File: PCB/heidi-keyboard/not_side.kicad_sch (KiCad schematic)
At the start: 65 parts, among them J1 USB_C_Receptacle_USB2.0_14P, J3 AudioJack4, SW1 SW_Push, SW11 SW_Push, SW13 SW_Push, SW14 SW_Push, SW15 SW_Push, SW16 SW_Push, SW17 SW_Push, SW18 SW_Push, SW25 SW_Push, SW26 SW_Push, SW27 SW_Push, SW28 SW_Push, SW29 SW_Push, SW3 SW_Push, SW30 SW_Push, SW37 SW_Push, SW38 SW_Push, SW39 SW_Push, SW40 SW_Push, SW41 SW_Push, SW42 SW_Push, SW49 SW_Push, SW5 SW_Push, SW50 SW_Push, SW51 SW_Push, SW52 SW_Push, SW53 SW_Push, SW54 SW_Push, SW7 SW_Push, SW9 SW_Push

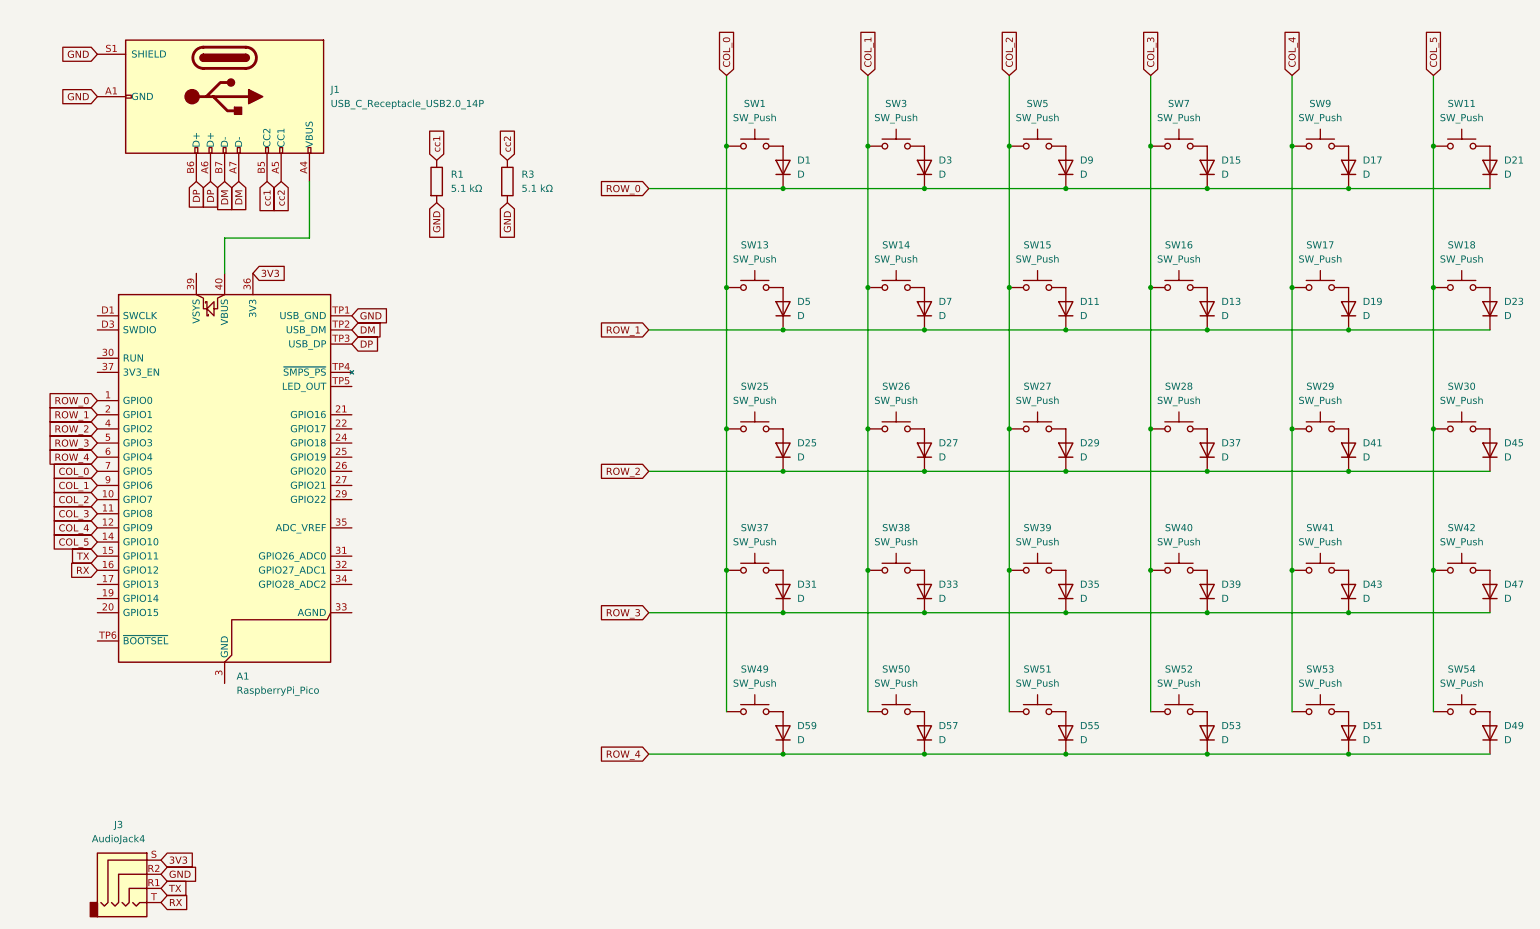
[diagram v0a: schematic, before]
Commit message: aaaaaaaaaaaaaaaaa
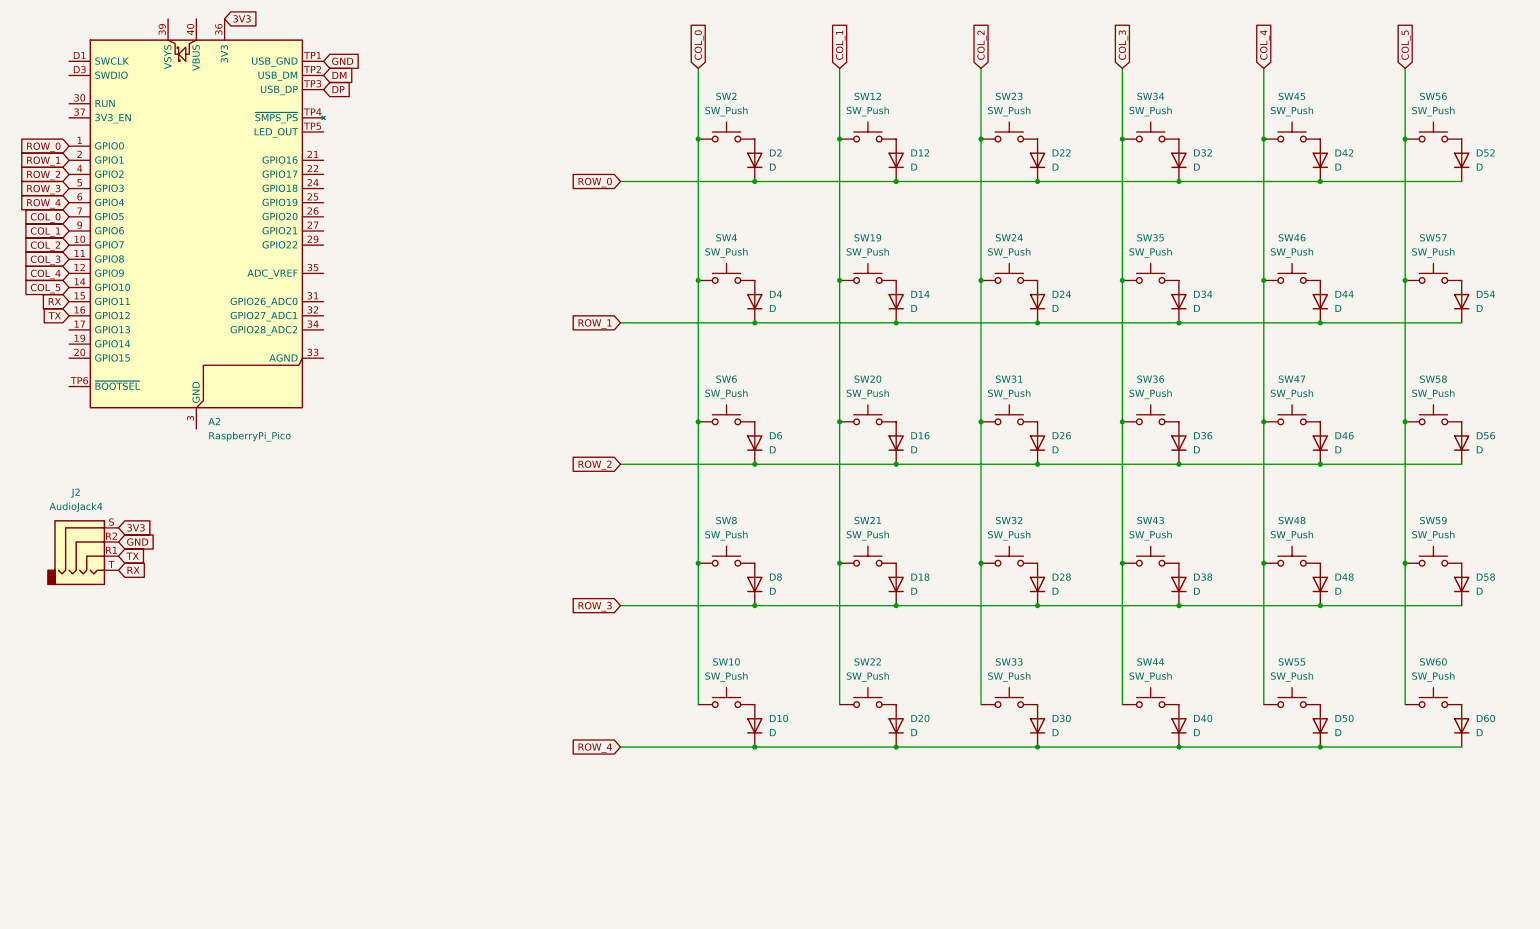
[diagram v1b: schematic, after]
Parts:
- removed A1: RaspberryPi_Pico, Module:RaspberryPi_Pico_SMD, symbol MCU_Module:RaspberryPi_Pico_Extensive
- removed D1, D11, D13, D15, D17, D19, D21, D23, D25, D27, D29, D3, D31, D33, D35, D37, D39, D41, D43, D45, D47, D49, D5, D51, D53, D55, D57, D59, D7, D9: D, symbol Device:D
- removed J1: USB_C_Receptacle_USB2.0_14P, symbol Connector:USB_C_Receptacle_USB2.0_14P
- removed J3: AudioJack4, symbol Connector_Audio:AudioJack4
- removed R1, R3: 5.1 kΩ, symbol Device:R
- removed SW1, SW11, SW13, SW14, SW15, SW16, SW17, SW18, SW25, SW26, SW27, SW28, SW29, SW3, SW30, SW37, SW38, SW39, SW40, SW41, SW42, SW49, SW5, SW50, SW51, SW52, SW53, SW54, SW7, SW9: SW_Push, symbol Switch:SW_Push
- added A2: RaspberryPi_Pico, Module:RaspberryPi_Pico_SMD, symbol MCU_Module:RaspberryPi_Pico_Extensive
- added D10, D12, D14, D16, D18, D2, D20, D22, D24, D26, D28, D30, D32, D34, D36, D38, D4, D40, D42, D44, D46, D48, D50, D52, D54, D56, D58, D6, D60, D8: D, symbol Device:D
- added J2: AudioJack4, symbol Connector_Audio:AudioJack4
- added SW10, SW12, SW19, SW2, SW20, SW21, SW22, SW23, SW24, SW31, SW32, SW33, SW34, SW35, SW36, SW4, SW43, SW44, SW45, SW46, SW47, SW48, SW55, SW56, SW57, SW58, SW59, SW6, SW60, SW8: SW_Push, symbol Switch:SW_Push
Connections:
- net 3V3: now also A2.36 (3V3), J2.S
- net COL_0: now also A2.7 (GPIO5), SW10.1, SW2.1, SW4.1, SW6.1, SW8.1
- net COL_1: now also A2.9 (GPIO6), SW12.1, SW19.1, SW20.1, SW21.1, SW22.1
- net COL_2: now also A2.10 (GPIO7), SW23.1, SW24.1, SW31.1, SW32.1, SW33.1
- net COL_3: now also A2.11 (GPIO8), SW34.1, SW35.1, SW36.1, SW43.1, SW44.1
- net COL_4: now also A2.12 (GPIO9), SW45.1, SW46.1, SW47.1, SW48.1, SW55.1
- net COL_5: now also A2.14 (GPIO10), SW56.1, SW57.1, SW58.1, SW59.1, SW60.1
- net DM: now also A2.TP2 (USB_DM)
- net DP: now also A2.TP3 (USB_DP)
- net GND: now also A2.TP1 (USB_GND), J2.R2
- net ROW_0: now also A2.1 (GPIO0), D12.1 (K), D2.1 (K), D22.1 (K), D32.1 (K), D42.1 (K), D52.1 (K)
- net ROW_1: now also A2.2 (GPIO1), D14.1 (K), D24.1 (K), D34.1 (K), D4.1 (K), D44.1 (K), D54.1 (K)
- net ROW_2: now also A2.4 (GPIO2), D16.1 (K), D26.1 (K), D36.1 (K), D46.1 (K), D56.1 (K), D6.1 (K)
- net ROW_3: now also A2.5 (GPIO3), D18.1 (K), D28.1 (K), D38.1 (K), D48.1 (K), D58.1 (K), D8.1 (K)
- net ROW_4: now also A2.6 (GPIO4), D10.1 (K), D20.1 (K), D30.1 (K), D40.1 (K), D50.1 (K), D60.1 (K)
- net RX: now also A2.15 (GPIO11), J2.T
- net TX: now also A2.16 (GPIO12), J2.R1
- new net: D22.2 (A), SW23.2
- new net: D44.2 (A), SW46.2
- new net: D4.2 (A), SW4.2
- new net: D26.2 (A), SW31.2
- new net: D16.2 (A), SW20.2
- new net: D32.2 (A), SW34.2
- new net: D28.2 (A), SW32.2
- new net: D20.2 (A), SW22.2
- new net: D8.2 (A), SW8.2
- new net: D6.2 (A), SW6.2
- new net: D12.2 (A), SW12.2
- new net: D36.2 (A), SW36.2
- new net: D30.2 (A), SW33.2
- new net: D54.2 (A), SW57.2
- new net: D24.2 (A), SW24.2
- new net: D60.2 (A), SW60.2
- new net: D18.2 (A), SW21.2
- new net: D10.2 (A), SW10.2
- new net: D50.2 (A), SW55.2
- new net: D34.2 (A), SW35.2
- new net: D58.2 (A), SW59.2
- new net: D38.2 (A), SW43.2
- new net: D52.2 (A), SW56.2
- new net: D42.2 (A), SW45.2
- new net: D46.2 (A), SW47.2
- new net: D14.2 (A), SW19.2
- new net: D48.2 (A), SW48.2
- new net: D56.2 (A), SW58.2
- new net: D2.2 (A), SW2.2
- new net: D40.2 (A), SW44.2
- new net: A2.13 (GND), A2.18 (GND), A2.23 (GND), A2.28 (GND), A2.3 (GND), A2.38 (GND), A2.8 (GND), A2.D2 (GND)

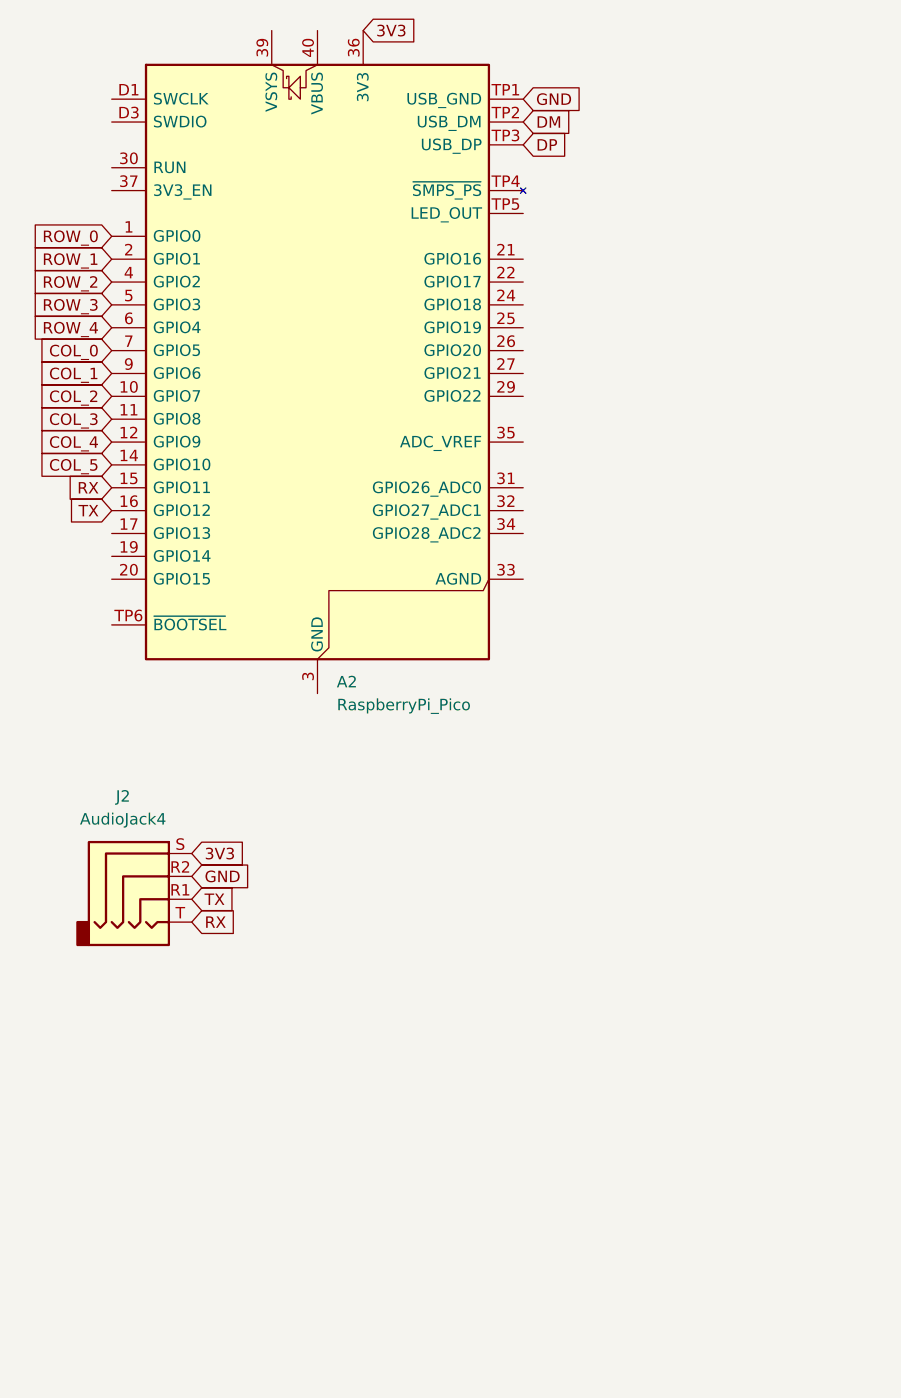
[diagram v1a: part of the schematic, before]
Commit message: aaaaaaaaaaaaaaaa
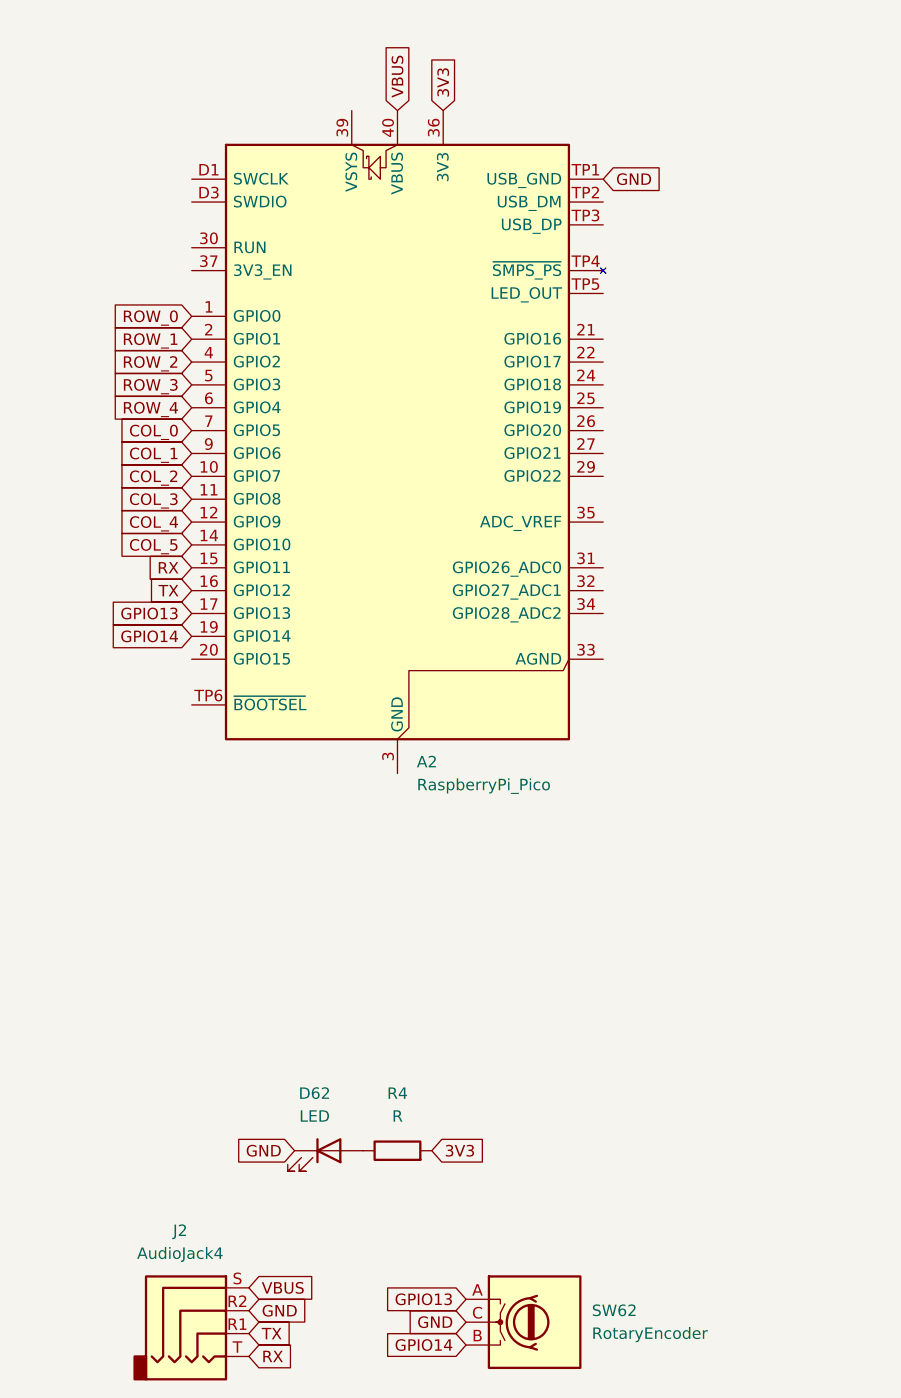
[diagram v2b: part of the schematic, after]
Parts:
- added D62: LED, symbol Device:LED
- added R4: R, symbol Device:R
- added SW62: RotaryEncoder, symbol Device:RotaryEncoder
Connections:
- net 3V3: now also R4.2; no longer J2.S
- net GND: now also D62.1 (K), SW62.C
- net GPIO13: now reaches A2.17 (GPIO13)
- net GPIO13: now also SW62.A
- net GPIO14: now reaches A2.19 (GPIO14)
- net GPIO14: now also SW62.B
- net VBUS: now reaches A2.40 (VBUS)
- net VBUS: now also J2.S
- net DM: no longer names the net of A2.TP2 (USB_DM)
- net DP: no longer names the net of A2.TP3 (USB_DP)
- new net: D62.2 (A), R4.1
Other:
- moved on the sheet: A2, J2
